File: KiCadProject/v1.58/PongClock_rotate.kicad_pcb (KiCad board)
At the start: 2 copper layers, 67.3 x 90.2 mm, 28 parts, among them J1 CONN_01X01_MALE, J2 MY_USB_OTG, SW1 SW_DIP_x01, SW2 SW_DIP_x01, U1 TinyRTC_I2C_RIGHT, U2 MAX7219_IN, U3 MAX7219_IN, U4 MAX7219_IN, U5 MAX7219_IN, U6 MAX7219_IN, U7 MAX7219_IN, U8 ATMEGA328P-PU, U9 FTDI1232, Y1 Crystal

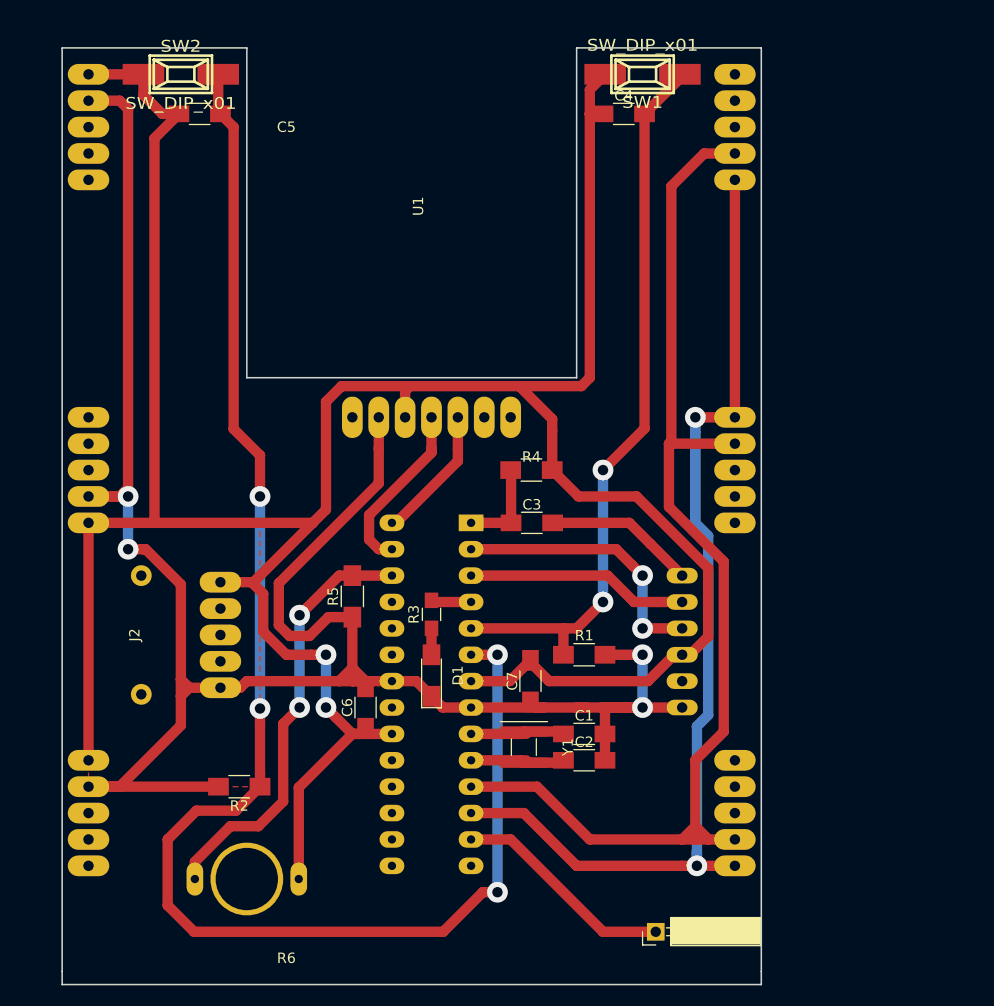
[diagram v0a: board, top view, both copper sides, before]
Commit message: v1.58
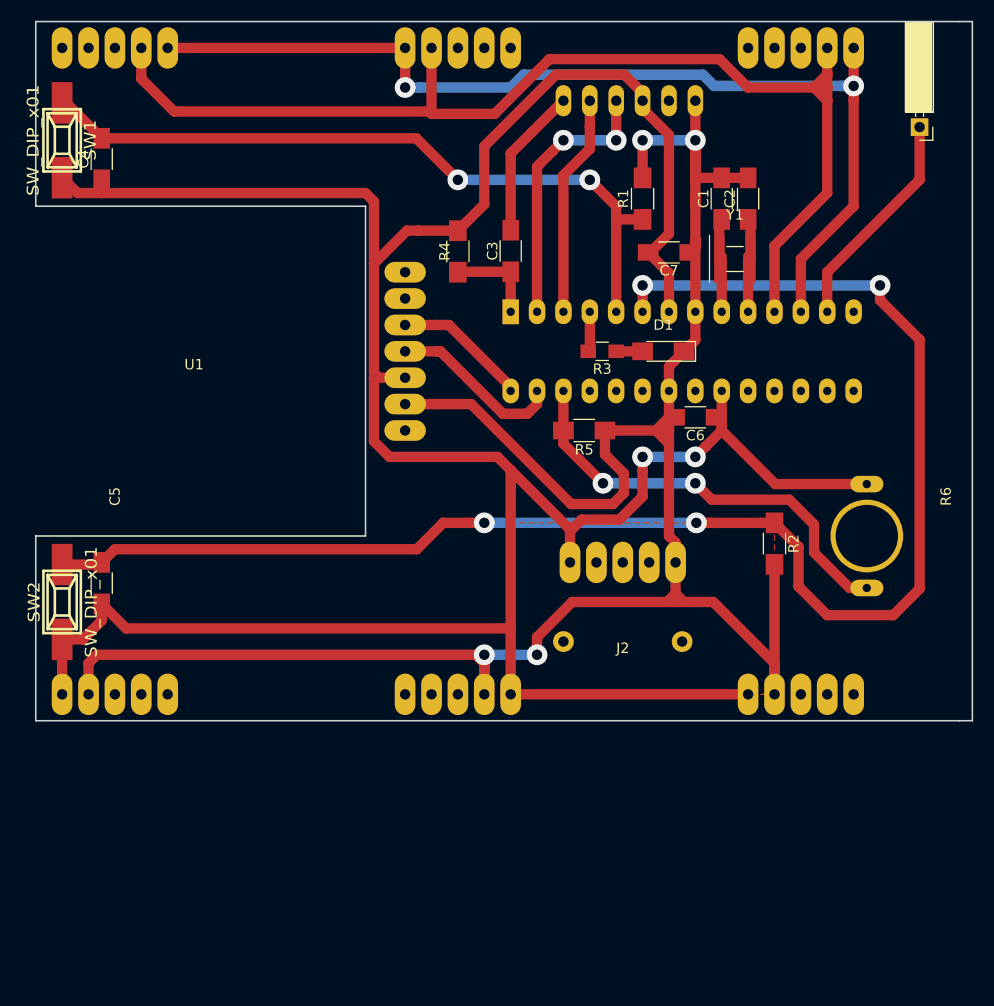
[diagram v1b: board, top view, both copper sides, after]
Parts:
- moved J1 81.5 mm to (191.8, 54.6), turned to 270 degrees
- moved U7 68.6 mm to (175.3, 47.0), turned to 270 degrees
- moved R6 68.2 mm to (186.7, 94.0), turned to 270 degrees
- moved U5 64.8 mm to (109.2, 47.0), turned to 270 degrees
- moved U4 63.8 mm to (175.3, 109.2), turned to 270 degrees
- moved U2 59.7 mm to (109.2, 109.2), turned to 270 degrees
- moved J2 59.5 mm to (173.4, 106.7), turned to 180 degrees
- moved R2 56.6 mm to (177.8, 94.7), turned to 270 degrees
- moved C2 56.3 mm to (175.3, 61.5), turned to 90 degrees
- moved SW1 56.2 mm to (109.2, 55.9), turned to 270 degrees
- moved C1 53.2 mm to (172.7, 61.5), turned to 90 degrees
- moved SW2 52.1 mm to (109.2, 100.3), turned to 90 degrees
- moved Y1 51.2 mm to (174.0, 67.3), turned to 0 degrees
- moved U6 50.6 mm to (152.4, 47.0), turned to 90 degrees
- moved C4 50.4 mm to (113.0, 57.7), turned to 90 degrees
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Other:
- board size 67.3 x 90.2 mm -> 90.2 x 67.3 mm
